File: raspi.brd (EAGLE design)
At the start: 60.6 x 53.3 mm, 5 parts

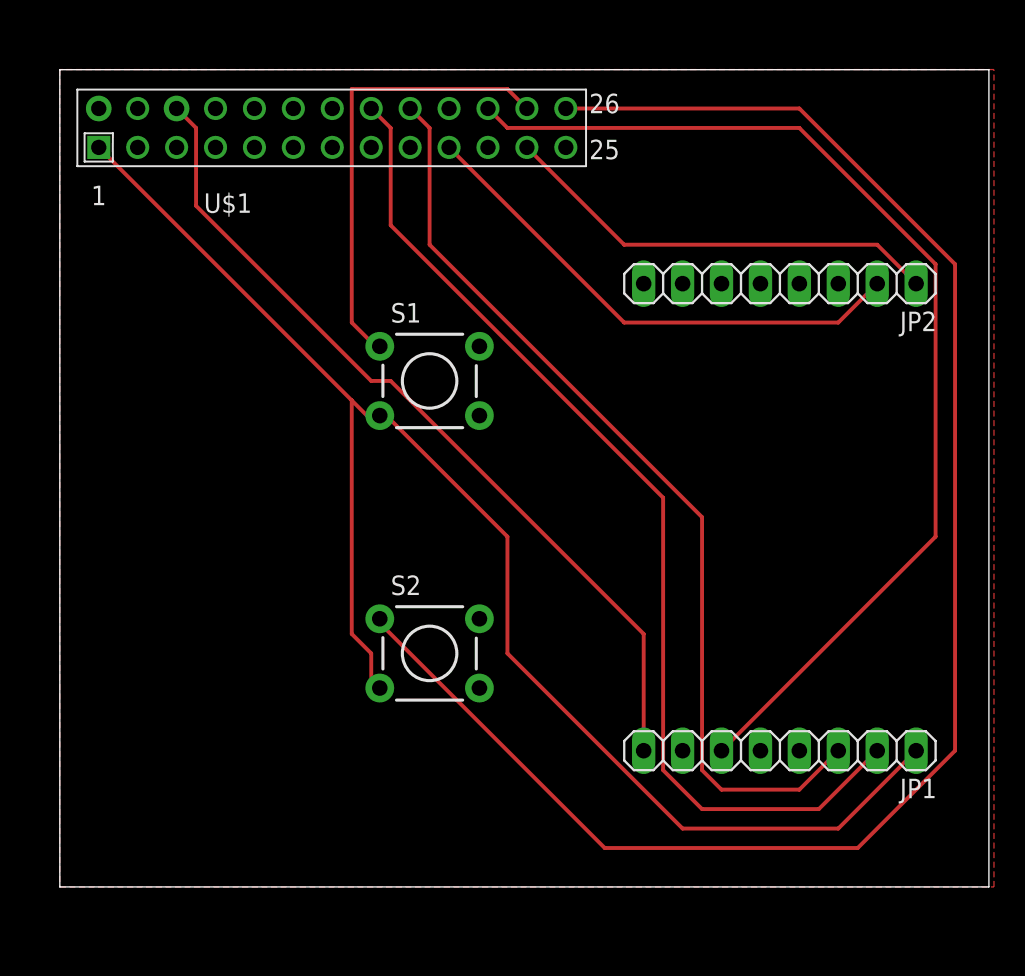
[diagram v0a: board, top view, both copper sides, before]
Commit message: work on shield
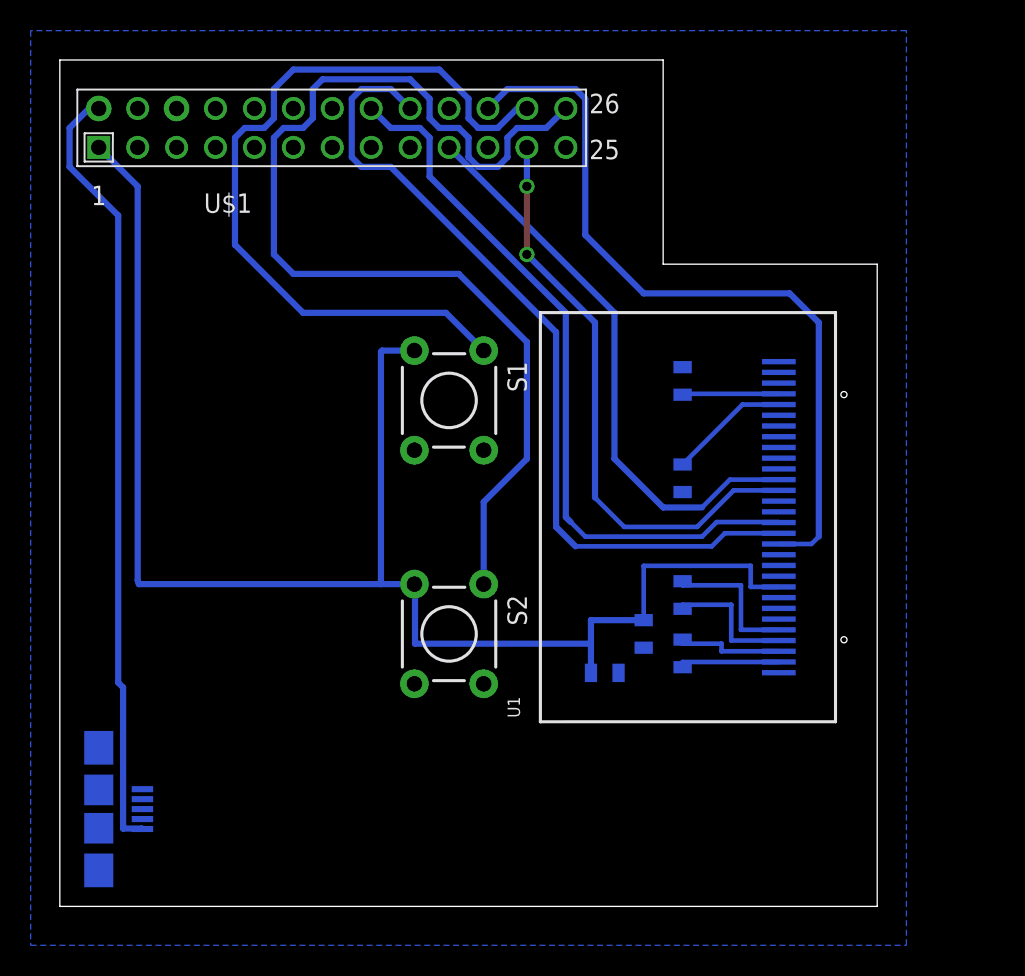
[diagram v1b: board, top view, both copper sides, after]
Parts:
- removed JP1, JP2: (no value), pinhead:1X08
- added C1, C2, C4, C5: 1uF, SparkFun-Capacitors:0805
- added C3: 104, SparkFun-Capacitors:0805
- added R1: 390k/560k, SparkFun-Resistors:0805
- added U$2: USB_AB, SparkFun-Connectors:USB-AB-MICRO-SMD
- added U1: (no value), microbuilder:UG-2864HSWEG01_0.96IN_WRAPAROUND
- S1, S2: value (none) -> SWITCH-MOMENTARY-2PTH; device SparkFun:TACTILE-PTH -> SparkFun-Electromechanical:TACTILE-PTH
- moved S1 1.80 mm to (25.4, 34.3), turned to 270 degrees
- moved S2 1.80 mm to (25.4, 19.1), turned to 270 degrees
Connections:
- new net +5V: U$1.2, U$2.VBUS
- new net N$1: U$1.19, U1.19
- new net N$10: C1.1, U1.2
- new net N$11: C2.1, U1.4
- new net N$12: C1.2, U1.3
- new net N$13: C2.2, U1.5
- new net N$4: U$1.16, U1.15
- new net VCC: U1.28
- new net VSS: U1.8
- net +3V3: now also C3.1, C4.1, U1.9; no longer JP1.1
- net GND: now also C3.2, C4.2, C5.2, R1.2, U$1.25, U$1.9, U$2.GND, U1.1, U1.10, U1.11, U1.12, U1.29, U1.30; no longer JP1.8
- net N$5: now also U1.18; no longer JP2.1
- net N$6: now also C5.1, U1.27; no longer JP2.2, U$1.19
- net N$7: now also U1.13; no longer JP1.6
- net N$8: now also U1.14; no longer JP1.3
- net N$9: now also R1.1, U1.26; no longer JP1.2, U$1.16
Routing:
- net N$9: track 67.7 -> 7.90 mm
- net GND: track 55.3 -> 0.00 mm
- net +5V: track 0.00 -> 50.9 mm
- net N$4: track 0.00 -> 47.9 mm
- net N$2: track 109.0 -> 71.4 mm
- net N$1: track 0.00 -> 37.6 mm
- net N$6: track 33.7 -> 6.30 mm
- net N$3: track 29.6 -> 50.9 mm
- net N$7: track 71.0 -> 50.4 mm
- net N$13: track 0.00 -> 9.45 mm
- net N$5: track 29.1 -> 38.5 mm, vias 0 -> 2
- net N$11: track 0.00 -> 8.88 mm
- net N$12: track 0.00 -> 7.04 mm
- net N$8: track 61.5 -> 54.6 mm
- net N$10: track 0.00 -> 6.62 mm
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- added copper zone on layer 16, net GND
- removed copper zone on layer 1, net GND
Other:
- board size 60.6 x 53.3 mm -> 53.3 x 55.2 mm
